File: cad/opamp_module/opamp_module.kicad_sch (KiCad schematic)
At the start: 20 parts, among them U1 REF3433IDBVR, U2 MCP34641R-E/ST, U4 OPA2325

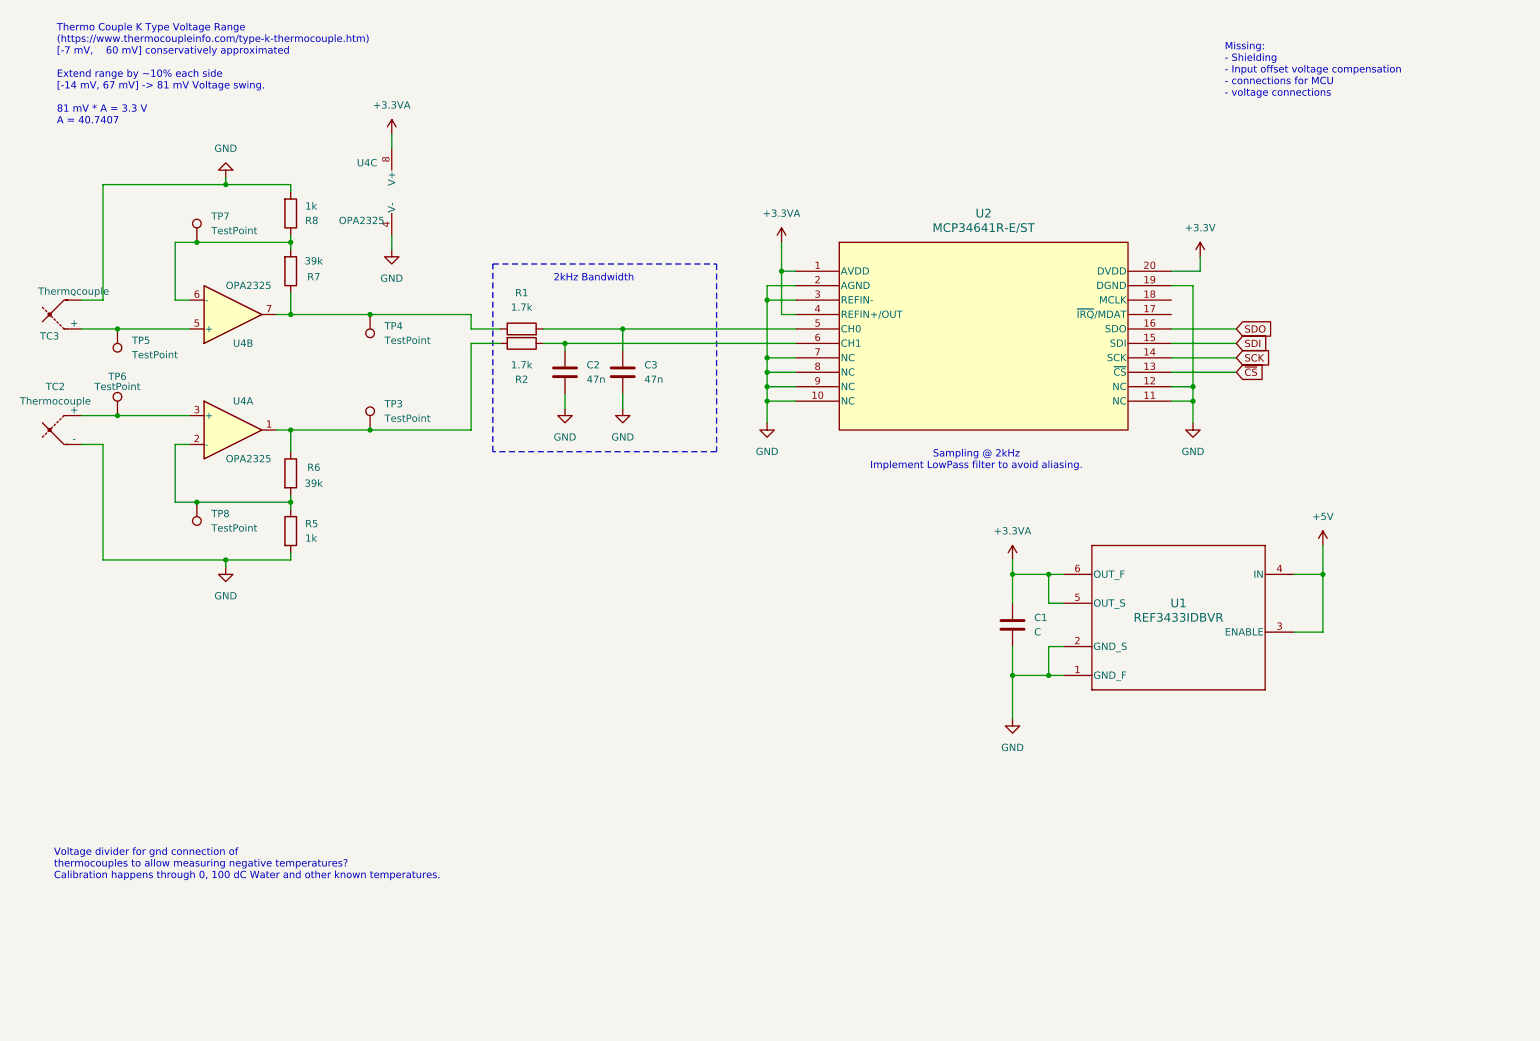
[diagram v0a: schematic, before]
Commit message: Spice based resistor selection :)
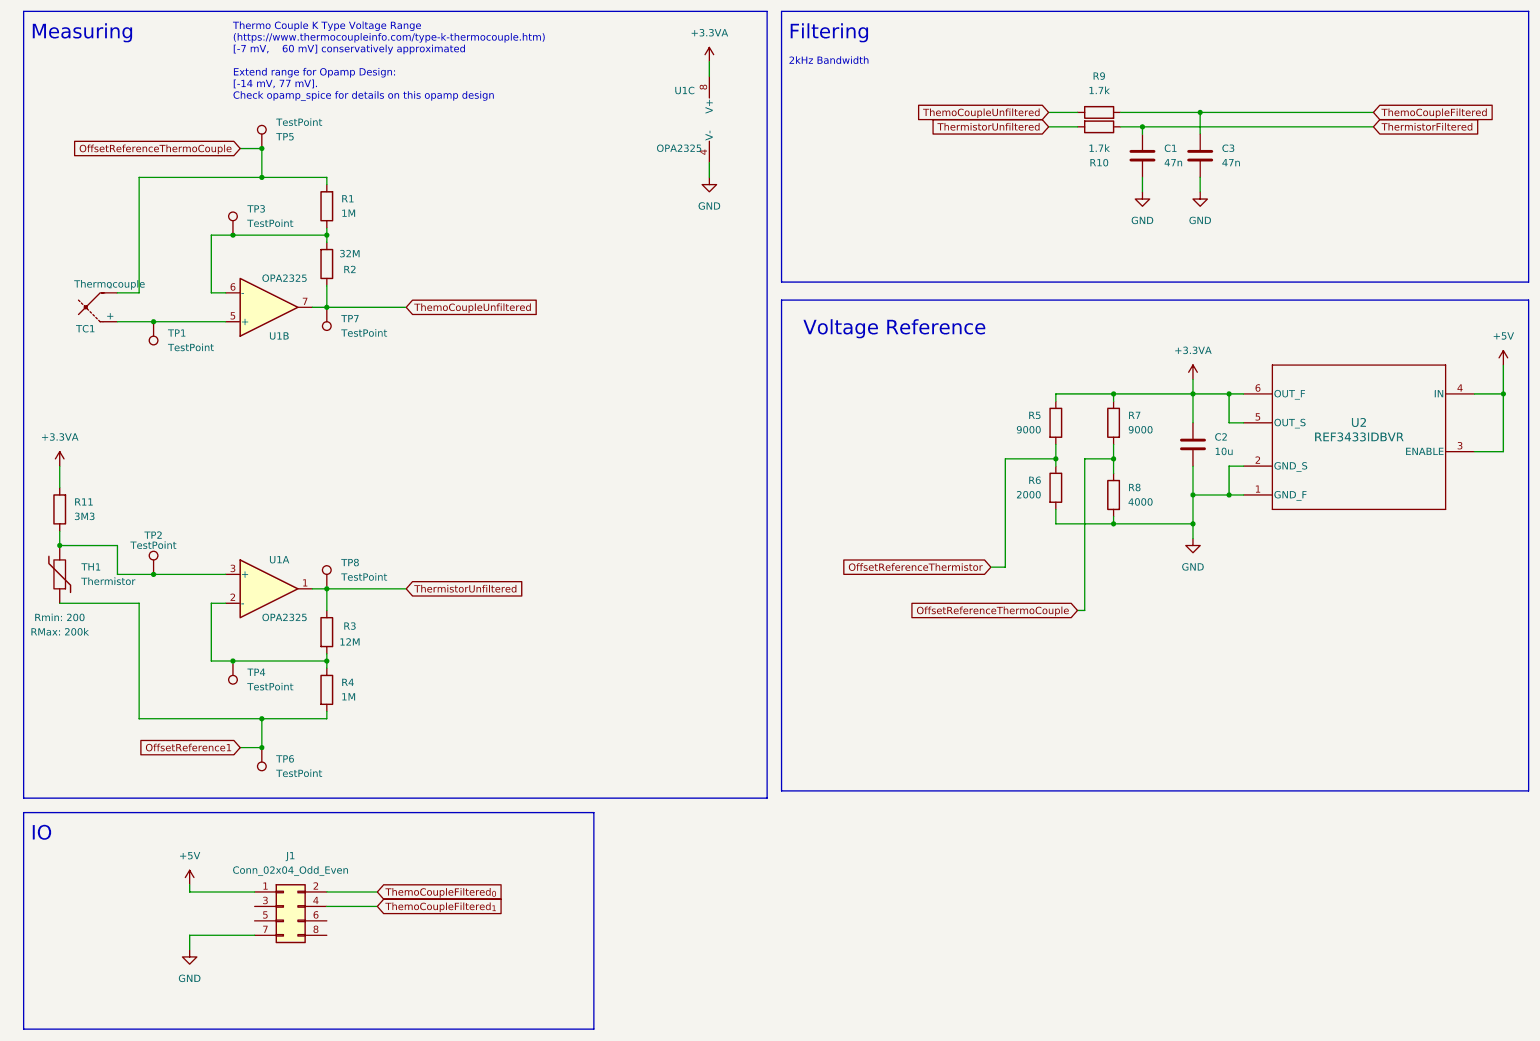
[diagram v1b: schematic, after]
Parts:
- removed TC2: Thermocouple, symbol Device:Thermocouple
- removed U2: MCP34641R-E/ST, TSSOP20_ST_MCH, symbol Library:MCP3461R-E/ST
- added J1: Conn_02x04_Odd_Even, symbol Connector_Generic:Conn_02x04_Odd_Even
- added R11: 3M3, symbol Device:R
- added R5, R7: 9000, symbol Device:R
- added R6: 2000, symbol Device:R
- added R8: 4000, symbol Device:R
- added TH1: Thermistor, symbol Device:Thermistor
- added TP5, TP6: TestPoint, symbol Connector:TestPoint
- C2: renamed from C1; value C -> 10u
- R1: renamed from R8; value 1k -> 1M
- R2: renamed from R7; value 39k -> 32M
- R3: renamed from R6; value 39k -> 12M
- R4: renamed from R5; value 1k -> 1M
- renumbered C2 to C1, R2 to R10, R1 to R9, TC3 to TC1, TP5 to TP1, TP6 to TP2, TP7 to TP3, TP8 to TP4, TP4 to TP7, TP3 to TP8, U4 to U1, U1 to U2
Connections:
- net +3.3VA: now also R11.2, R5.1, R7.1
- net +5V: now also J1.1 (Pin_1)
- net GND: now also J1.7 (Pin_7), R6.2, R8.2; no longer R1.2, R4.2, TC1.2 (-)
- net ThemoCoupleFiltered: now reaches C3.1, R9.2
- net ThermistorFiltered: now reaches C1.1, R10.1
- net ThemoCoupleUnfiltered: now reaches R2.1, R9.1, TP7.1, U1.7
- net ThermistorUnfiltered: now reaches R10.2, R3.1, TP8.1, U1.1
- net at TP2.1, U1.3 (+): now also R11.1, TH1.2
- new net OffsetReference1: R4.2, TH1.1, TP6.1
- new net OffsetReferenceThermistor: R5.2, R6.1
- new net OffsetReferenceThermoCouple: R1.2, R7.2, R8.1, TC1.2 (-), TP5.1
- new net ThemoCoupleFiltered_{0}: J1.2 (Pin_2)
- new net ThemoCoupleFiltered_{1}: J1.4 (Pin_4)
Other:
- note added: "Filtering"
- note added: "IO"
- note added: "Measuring"
- note added: "Thermo Couple K Type Voltage Range (https://www.thermocoupleinfo.com/type-k-thermocouple.htm) [-7 mV, 60 mV] conservatively approximated Extend range for Opamp Design: [-14 mV, 77 mV]. Check opamp_spice for details on this opamp design"
- note added: "Voltage Reference"
- note removed: "Missing: - Shielding - Input offset voltage compensation - connections for MCU - voltage connections"
- note removed: "Sampling @ 2kHz Implement LowPass filter to avoid aliasing."
- note removed: "Thermo Couple K Type Voltage Range (https://www.thermocoupleinfo.com/type-k-thermocouple.htm) [-7 mV, 60 mV] conservatively approximated Extend range by ~10% each side [-14 mV, 67 mV] -> 81 mV Voltage swing. 81 mV * A = 3.3 V A = 40.7407"
- note removed: "Voltage divider for gnd connection of thermocouples to allow measuring negative temperatures? Calibration happens through 0, 100 dC Water and other known temperatures."
- moved on the sheet: C1, C2, C3, R1, R10, R2, R3, R4, R9, TC1, TP1, TP2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
